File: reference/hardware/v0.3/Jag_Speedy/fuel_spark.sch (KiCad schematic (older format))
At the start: 73 parts, among them IC3 VNLD5090-E, IC4 VNLD5090-E, IC5 VNLD5090-E, IC6 TC4424EPA, IC7 TC4424EPA, IC8 TC4424EPA

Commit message: Schematic pin mapping
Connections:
- net labels added: Ign01-Trigger, Ign02-Trigger, Ign03-Trigger, Ign04-Trigger, Ign05-Trigger, Ign06-Trigger, Inj01-Trigger, Inj02-Trigger, Inj03-Trigger, Inj04-Trigger, Inj05-Trigger, Inj06-Trigger
- net labels removed: Ign01-CPU-D39, Ign02-CPU-D38, Ign03-CPU-D31, Ign04-CPU-D21, Ign05-CPU-D32, Ign06-CPU-D35, Inj01-CPU-D08, Inj02-CPU-D09, Inj03-CPU-D10, Inj04-CPU-D11, Inj05-CPU-D12, Inj06-CPU-D07
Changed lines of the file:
@@
 $EndComp
 Text GLabel 7700 1650 0    50   Input ~ 0
-Ign01-CPU-D39
+Ign01-Trigger
 Text GLabel 7700 1850 0    50   Input ~ 0
-Ign02-CPU-D38
+Ign02-Trigger
 Text GLabel 9800 1200 2    50   Output ~ 0
 Ign01-OUT
@@
 $EndComp
 Text GLabel 7750 3600 0    50   Input ~ 0
-Ign03-CPU-D31
+Ign03-Trigger
 Text GLabel 7750 3800 0    50   Input ~ 0
-Ign04-CPU-D21
+Ign04-Trigger
 Text GLabel 9850 3150 2    50   Output ~ 0
 Ign03-OUT
@@
 $EndComp
 Text GLabel 7750 5550 0    50   Input ~ 0
-Ign05-CPU-D32
+Ign05-Trigger
 Text GLabel 7750 5750 0    50   Input ~ 0
-Ign06-CPU-D35
+Ign06-Trigger
 Text GLabel 9850 5100 2    50   Output ~ 0
 Ign05-OUT
@@
 $EndComp
 Text GLabel 1250 1650 0    50   Input ~ 0
-Inj02-CPU-D09
+Inj02-Trigger
 $Comp
 L Device:R R44
@@
 $EndComp
 Text GLabel 1250 1450 0    50   Input ~ 0
-Inj01-CPU-D08
+Inj01-Trigger
 $Comp
 L VNLD5090-E:VNLD5090-E IC3
@@
 $EndComp
 Text GLabel 1250 3800 0    50   Input ~ 0
-Inj03-CPU-D10
+Inj03-Trigger
 Text GLabel 3900 3400 2    50   Output ~ 0
 Inj03-OUT
 Text GLabel 1250 4000 0    50   Input ~ 0
-Inj04-CPU-D11
+Inj04-Trigger
 Text GLabel 3900 4500 2    50   Output ~ 0
 Inj04-OUT
@@
 $EndComp
 Text GLabel 1250 6000 0    50   Input ~ 0
-Inj05-CPU-D12
+Inj05-Trigger
 Text GLabel 1250 6200 0    50   Input ~ 0
-Inj06-CPU-D07
+Inj06-Trigger
 Text GLabel 3900 5600 2    50   Output ~ 0
 Inj05-OUT

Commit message: Driver replacement
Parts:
- added IC?: VNS3NV04DP-E, SOIC127P600X175-8N, symbol VNS3NV04DP-E:VNS3NV04DP-E
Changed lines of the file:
@@
 Text GLabel 3900 2150 2    50   Output ~ 0
 Inj02-OUT
+$Comp
+L VNS3NV04DP-E:VNS3NV04DP-E IC?
+U 1 1 5F28A4DE
+P -2600 1500
+F 0 "IC?" H -1800 1765 50  0000 C CNN
+F 1 "VNS3NV04DP-E" H -1800 1674 50  0000 C CNN
+F 2 "SOIC127P600X175-8N" H -1150 1600 50  0001 L CNN
+F 3 "https://www.st.com/resource/en/datasheet/vns3nv04dp-e.pdf" H -1150 1500 50  0001 L CNN
+F 4 "STMicroelectronics VNS3NV04DP-E Load Switch IC, 8-Pin, SOIC" H -1150 1400 50  0001 L CNN "Description"
+F 5 "1.75" H -1150 1300 50  0001 L CNN "Height"
+F 6 "STMicroelectronics" H -1150 1200 50  0001 L CNN "Manufacturer_Name"
+F 7 "VNS3NV04DP-E" H -1150 1100 50  0001 L CNN "Manufacturer_Part_Number"
+F 8 "VNS3NV04DP-E" H -1150 1000 50  0001 L CNN "Arrow Part Number"
+F 9 "https://www.arrow.com/en/products/vns3nv04dp-e/stmicroelectronics" H -1150 900 50  0001 L CNN "Arrow Price/Stock"
+F 10 "511-VNS3NV04DP-E" H -1150 800 50  0001 L CNN "Mouser Part Number"
+F 11 "https://www.mouser.com/Search/Refine.aspx?Keyword=511-VNS3NV04DP-E" H -1150 700 50  0001 L CNN "Mouser Price/Stock"
+	1    -2600 1500
+	1    0    0    -1
+$EndComp
 $EndSCHEMATC

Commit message: MOSFET Drivers
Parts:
- removed IC3, IC4, IC5: VNLD5090-E, Package_SO:SO-8_5.3x6.2mm_P1.27mm, symbol VNLD5090-E:VNLD5090-E
- added IC4, IC5: VNS3NV04DP-E, SOIC127P600X175-8N, symbol Jag_Speedy-rescue:VNS3NV04DP-E-VNS3NV04DP-E
- IC3: renamed from IC?; symbol VNS3NV04DP-E:VNS3NV04DP-E -> Jag_Speedy-rescue:VNS3NV04DP-E-VNS3NV04DP-E
- IC6, IC7, IC8: symbol TC4424EPA:TC4424EPA -> Jag_Speedy-rescue:TC4424EPA-TC4424EPA
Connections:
- wire segments 105 -> 123
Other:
- note added: "Injector 01 & 02"
- note added: "Injector 03 & 04"
- note added: "Injector 05 & 06"
- note removed: "Injector 01 (D08) & 02 (D09)"
- note removed: "Injector 03 (D10) & 04 (D11)"
- note removed: "Injector 05 (D12) & 06 (D07)"

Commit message: Rationalise level shifting
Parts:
- IC3, IC4, IC5: footprint SOIC127P600X175-8N -> Package_SO:SO-8_3.9x4.9mm_P1.27mm; symbol Jag_Speedy-rescue:VNS3NV04DP-E-VNS3NV04DP-E -> Jag_Speedy-rescue:VNS3NV04DP-E-VNS3NV04DP-E-Jag_Speedy-rescue
- IC6, IC7, IC8: symbol Jag_Speedy-rescue:TC4424EPA-TC4424EPA -> Jag_Speedy-rescue:TC4424EPA-TC4424EPA-Jag_Speedy-rescue
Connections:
- net Inj03-Trigger: now also R40.1; no longer R40.2
- net SignalGnd: now also R40.2; no longer R40.1
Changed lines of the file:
@@
 Injector 05 & 06
 $Comp
-L Jag_Speedy-rescue:TC4424EPA-TC4424EPA IC6
+L Jag_Speedy-rescue:TC4424EPA-TC4424EPA-Jag_Speedy-rescue IC6
 U 1 1 5F1EF1D7
 P 8200 1550
@@
 Wire Wire Line
 	9200 1200 8750 1200
-Text GLabel 7700 1200 0    50   Input ~ 0
-PowerGnd
 Wire Wire Line
 	7700 1200 7750 1200
@@
 Wire Wire Line
 	7700 1750 8200 1750
-Text GLabel 7700 2250 0    50   Input ~ 0
-PowerGnd
 Connection ~ 7750 1850
 Wire Wire Line
@@
 	9500 1850 9500 2250
 $Comp
-L Jag_Speedy-rescue:TC4424EPA-TC4424EPA IC7
+L Jag_Speedy-rescue:TC4424EPA-TC4424EPA-Jag_Speedy-rescue IC7
 U 1 1 5F0F7B19
 P 8250 3500
@@
 Wire Wire Line
 	9250 3150 8800 3150
-Text GLabel 7750 3150 0    50   Input ~ 0
-PowerGnd
 Wire Wire Line
 	7750 3150 7800 3150
@@
 Wire Wire Line
 	7750 3700 8250 3700
-Text GLabel 7750 4200 0    50   Input ~ 0
-PowerGnd
 Connection ~ 7800 3800
 Wire Wire Line
@@
 	9550 3800 9550 4200
 $Comp
-L Jag_Speedy-rescue:TC4424EPA-TC4424EPA IC8
+L Jag_Speedy-rescue:TC4424EPA-TC4424EPA-Jag_Speedy-rescue IC8
 U 1 1 5F10DC80
 P 8250 5450
@@
 Wire Wire Line
 	9250 5100 8800 5100
-Text GLabel 7750 5100 0    50   Input ~ 0
-PowerGnd
 Wire Wire Line
 	7750 5100 7800 5100
@@
 Wire Wire Line
 	7750 5650 8250 5650
-Text GLabel 7750 6150 0    50   Input ~ 0
-PowerGnd
 Connection ~ 7800 5750
 Wire Wire Line
@@
 NoConn ~ 9450 5450
 $Comp
-L Jag_Speedy-rescue:VNS3NV04DP-E-VNS3NV04DP-E IC3
+L Jag_Speedy-rescue:VNS3NV04DP-E-VNS3NV04DP-E-Jag_Speedy-rescue IC3
 U 1 1 5F28A4DE
 P 2150 1650
 F 0 "IC3" H 2950 1915 50  0000 C CNN
 F 1 "VNS3NV04DP-E" H 2950 1824 50  0000 C CNN
-F 2 "SOIC127P600X175-8N" H 3600 1750 50  0001 L CNN
+F 2 "Package_SO:SO-8_3.9x4.9mm_P1.27mm" H 3600 1750 50  0001 L CNN
 F 3 "https://www.st.com/resource/en/datasheet/vns3nv04dp-e.pdf" H 3600 1650 50  0001 L CNN
 F 4 "STMicroelectronics VNS3NV04DP-E Load Switch IC, 8-Pin, SOIC" H 3600 1550 50  0001 L CNN "Description"
@@
 	1350 1950 1450 1950
 $Comp
-L Jag_Speedy-rescue:VNS3NV04DP-E-VNS3NV04DP-E IC4
+L Jag_Speedy-rescue:VNS3NV04DP-E-VNS3NV04DP-E-Jag_Speedy-rescue IC4
 U 1 1 5F0265BB
 P 2150 3850
 F 0 "IC4" H 2950 4115 50  0000 C CNN
 F 1 "VNS3NV04DP-E" H 2950 4024 50  0000 C CNN
-F 2 "SOIC127P600X175-8N" H 3600 3950 50  0001 L CNN
+F 2 "Package_SO:SO-8_3.9x4.9mm_P1.27mm" H 3600 3950 50  0001 L CNN
 F 3 "https://www.st.com/resource/en/datasheet/vns3nv04dp-e.pdf" H 3600 3850 50  0001 L CNN
 F 4 "STMicroelectronics VNS3NV04DP-E Load Switch IC, 8-Pin, SOIC" H 3600 3750 50  0001 L CNN "Description"
@@
 F 3 "~" H 1350 3700 50  0001 C CNN
 	1    1350 3700
-	1    0    0    -1
+	-1   0    0    1
 $EndComp
 $Comp
@@
 	1350 4150 1450 4150
 $Comp
-L Jag_Speedy-rescue:VNS3NV04DP-E-VNS3NV04DP-E IC5
+L Jag_Speedy-rescue:VNS3NV04DP-E-VNS3NV04DP-E-Jag_Speedy-rescue IC5
 U 1 1 5F03E989
 P 2150 6150
 F 0 "IC5" H 2950 6415 50  0000 C CNN
 F 1 "VNS3NV04DP-E" H 2950 6324 50  0000 C CNN
-F 2 "SOIC127P600X175-8N" H 3600 6250 50  0001 L CNN
+F 2 "Package_SO:SO-8_3.9x4.9mm_P1.27mm" H 3600 6250 50  0001 L CNN
 F 3 "https://www.st.com/resource/en/datasheet/vns3nv04dp-e.pdf" H 3600 6150 50  0001 L CNN
 F 4 "STMicroelectronics VNS3NV04DP-E Load Switch IC, 8-Pin, SOIC" H 3600 6050 50  0001 L CNN "Description"
@@
 NoConn ~ 3750 6150
 NoConn ~ 3750 6350
+Text GLabel 7750 6150 0    50   Input ~ 0
+PowerGnd
+Text GLabel 7750 5100 0    50   Input ~ 0
+PowerGnd
+Text GLabel 7750 4200 0    50   Input ~ 0
+PowerGnd
+Text GLabel 7750 3150 0    50   Input ~ 0
+PowerGnd
+Text GLabel 7700 2250 0    50   Input ~ 0
+PowerGnd
+Text GLabel 7700 1200 0    50   Input ~ 0
+PowerGnd
 $EndSCHEMATC

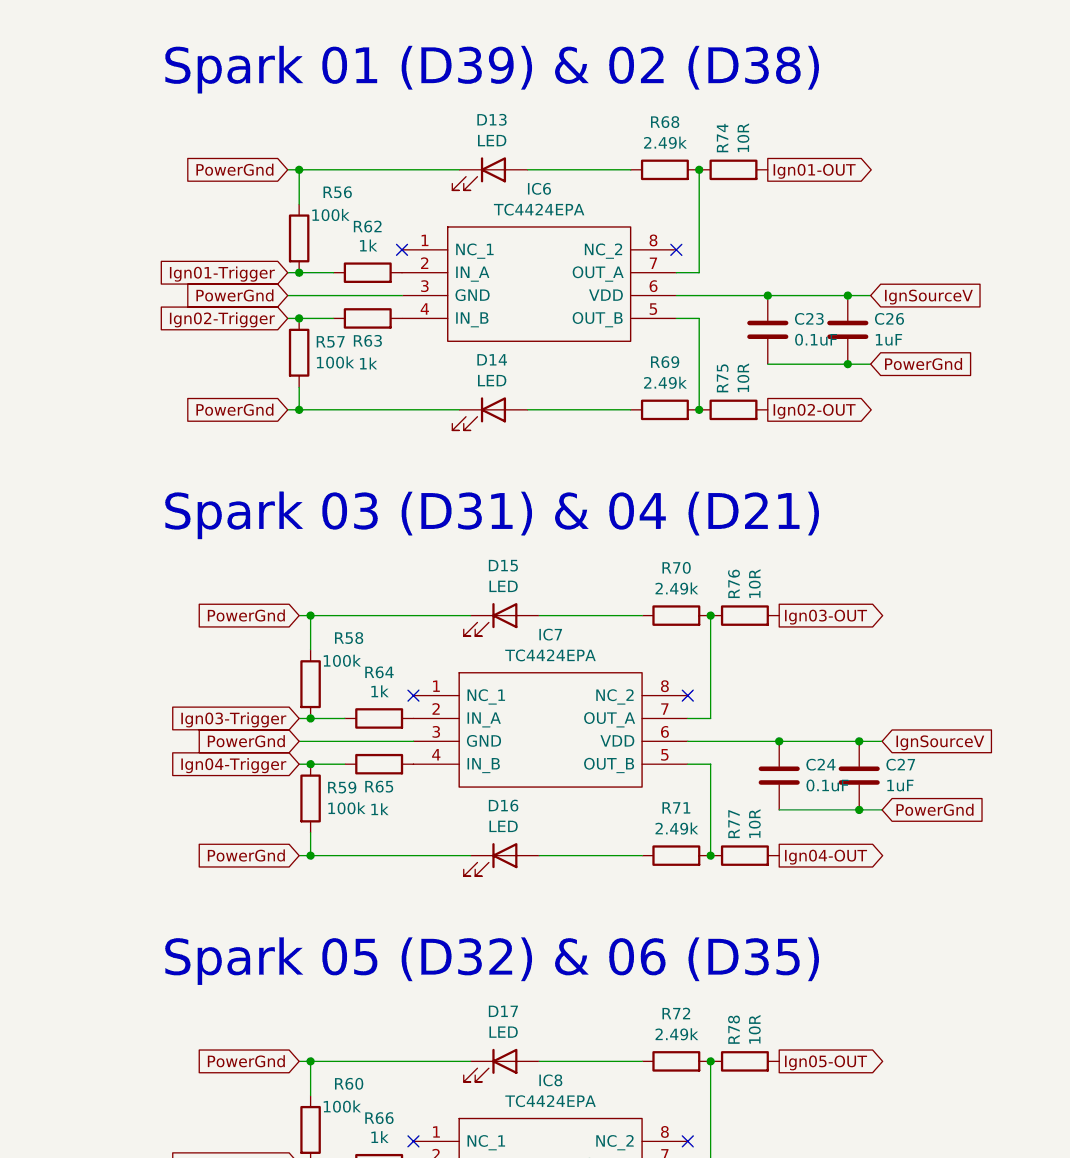
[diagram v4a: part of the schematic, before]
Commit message: Schematic tidyup
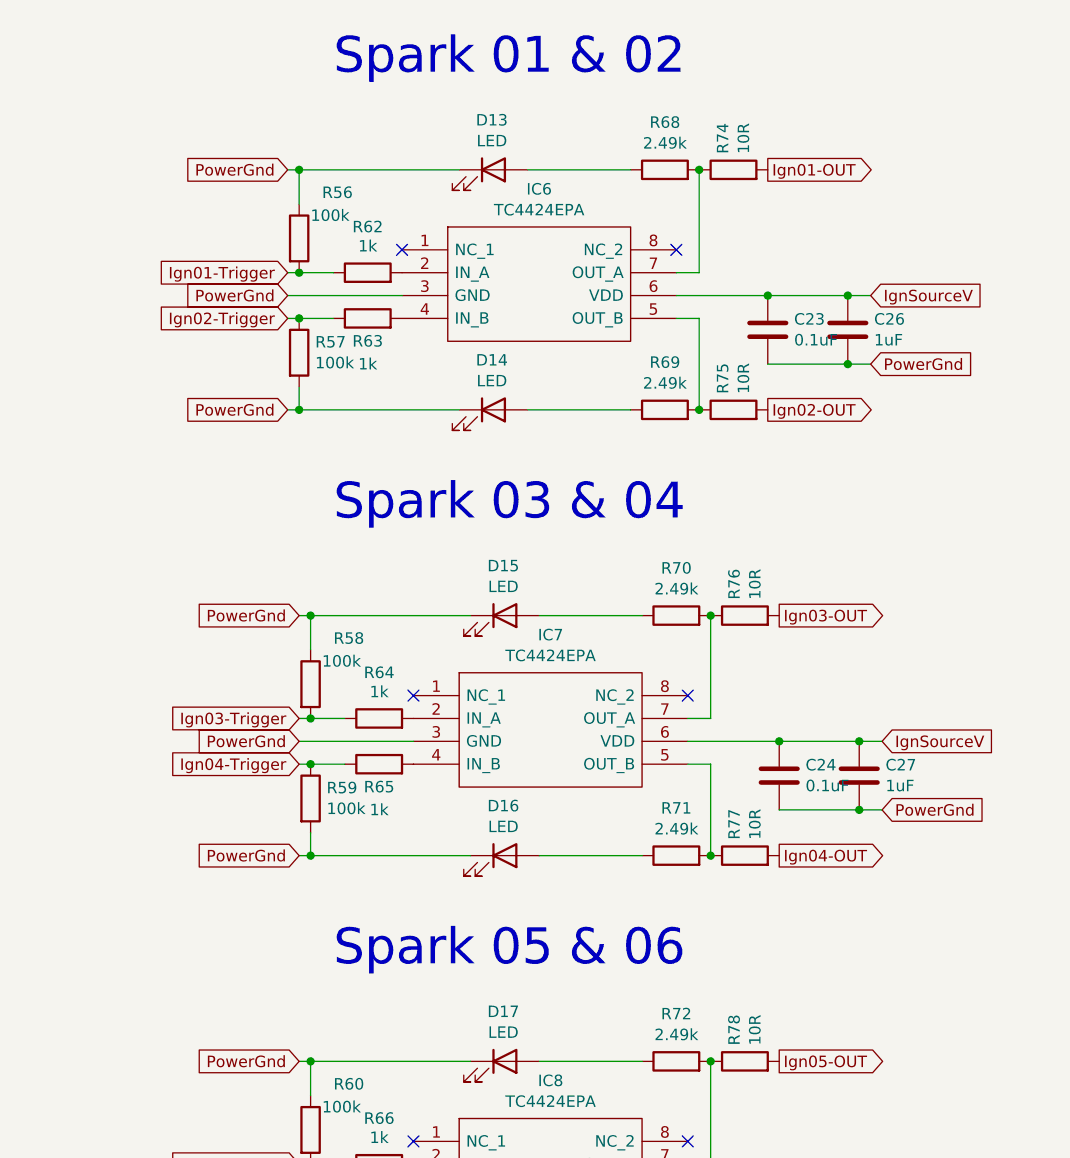
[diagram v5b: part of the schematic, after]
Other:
- note added: "Spark 01 & 02"
- note added: "Spark 03 & 04"
- note added: "Spark 05 & 06"
- note removed: "Spark 01 (D39) & 02 (D38)"
- note removed: "Spark 03 (D31) & 04 (D21)"
- note removed: "Spark 05 (D32) & 06 (D35)"
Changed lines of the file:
@@
 	9800 1750 9400 1750
 Connection ~ 9800 1750
-Text Notes 7150 850  0    157  ~ 0
-Spark 01 (D39) & 02 (D38)
-Text Notes 7150 2800 0    157  ~ 0
-Spark 03 (D31) & 04 (D21)
-Text Notes 7150 4750 0    157  ~ 0
-Spark 05 (D32) & 06 (D35)
+Text Notes 7900 800  0    157  ~ 0
+Spark 01 & 02
+Text Notes 7900 2750 0    157  ~ 0
+Spark 03 & 04
+Text Notes 7900 4700 0    157  ~ 0
+Spark 05 & 06
 Wire Wire Line
 	9800 1750 10150 1750

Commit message: SMD Update
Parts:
- C23, C24, C25, C26, C27, C28: footprint Capacitor_THT:CP_Radial_D5.0mm_P2.50mm -> Capacitor_SMD:C_0805_2012Metric
- D1, D13, D14, D15, D16, D17, D18, D2, D3, D4, D5, D6: footprint LED_THT:LED_D3.0mm -> LED_SMD:LED_0805_2012Metric
- D10, D11, D12, D7, D8, D9: footprint Diode_THT:D_DO-41_SOD81_P10.16mm_Horizontal -> Diode_SMD:D_SOD-323
- IC6, IC7, IC8: footprint Package_DIP:DIP-10_W7.62mm -> Package_SO:SOIC-8_3.9x4.9mm_P1.27mm
- R38, R39, R40, R41, R42, R43, R44, R45, R46, R47, R48, R49, R50, R51, R52, R53, R54, R55, R56, R57, R58, R59, R60, R61, R62, R63, R64, R65, R66, R67, R68, R69, R70, R71, R72, R73, R74, R75, R76, R77, R78, R79: footprint Resistor_THT:R_Axial_DIN0207_L6.3mm_D2.5mm_P2.54mm_Vertical -> Resistor_SMD:R_0805_2012Metric
